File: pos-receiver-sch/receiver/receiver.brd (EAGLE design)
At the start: 100 x 80 mm, 19 parts, among them IC1 AD8599R, IC2 78L10F

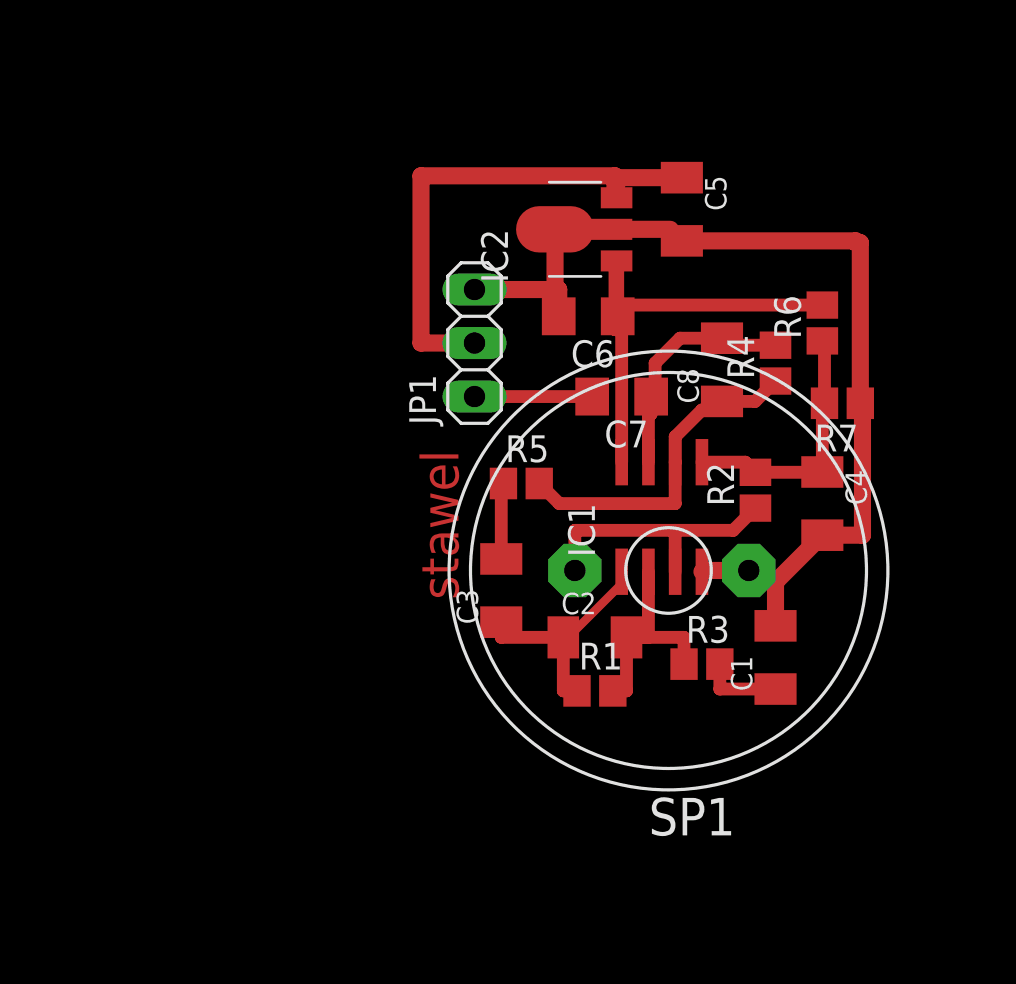
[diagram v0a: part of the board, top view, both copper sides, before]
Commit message: charge amp
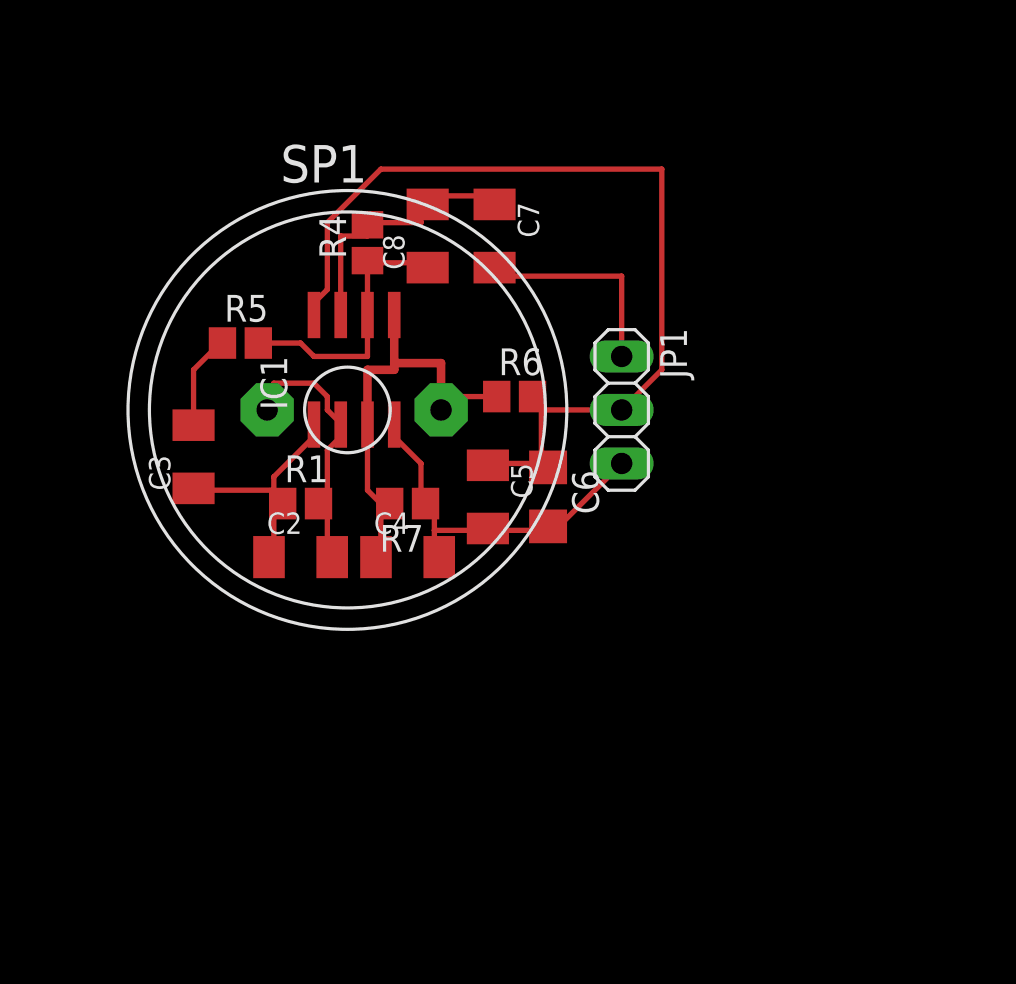
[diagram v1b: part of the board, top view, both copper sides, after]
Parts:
- removed C1: 10n, resistor:C1206K
- removed IC2: 78L10F, linear:SOT89
- removed R2: 200k, resistor:R0805
- removed R3: 3.3k, resistor:R0805
- C7: device resistor:C1206 -> resistor:C1206K
- moved R7 21.2 mm to (36.8, 22.9)
- moved R4 20.2 mm to (34.9, 35.2)
- moved C4 19.8 mm to (36.8, 20.3), turned to 0 degrees
- moved SP1 17.0 mm to (34.0, 27.3), turned to 0 degrees
- moved R1 16.6 mm to (31.8, 22.9)
- moved C5 16.5 mm to (40.6, 23.2)
- moved IC1 16.2 mm to (34.3, 29.2)
- moved C3 15.9 mm to (26.7, 25.1)
- moved C8 15.3 mm to (37.8, 35.6)
- moved R6 15.0 mm to (41.9, 27.9), turned to 0 degrees
- moved R5 14.9 mm to (28.9, 30.5)
- moved C2 14.5 mm to (31.8, 20.3)
- moved C7 9.72 mm to (41.0, 35.6), turned to 270 degrees
- moved C6 8.78 mm to (43.5, 23.2), turned to 270 degrees
- moved JP1 7.67 mm to (47.0, 27.3), turned to 270 degrees
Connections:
- removed net N$10: C5.1, IC2.3, JP1.2
- removed net N$2: C2.2, IC1.2, R1.2, R3.1
- removed net N$7: IC1.3, R2.1, SP1.2
- net GND: no longer C1.2, IC2.2, IC2.2@1, SP1.1
- net N$3: now also C2.2, IC1.2, R1.2, SP1.1; no longer C1.1, R3.2
- net N$9: now also IC1.3, SP1.2; no longer R2.2
- net VCC: now also C5.1, JP1.2; no longer IC2.1
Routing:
- net GND: track 47.9 -> 18.1 mm
- net N$10: track 24.9 -> 0.00 mm
- net VCC: track 24.4 -> 45.0 mm
- net N$7: track 12.9 -> 0.00 mm
- net N$2: track 11.3 -> 0.00 mm
- net N$3: track 3.82 -> 13.2 mm
- net N$9: track 12.2 -> 21.4 mm
- net N$1: track 5.59 -> 10.0 mm
- net N$4: track 15.9 -> 12.9 mm
- net N$5: track 11.2 -> 12.8 mm
- net N$8: track 11.3 -> 12.4 mm
- net N$6: track 3.62 -> 4.53 mm
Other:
- board text removed: "stawel"
